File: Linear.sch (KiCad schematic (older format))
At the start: 61 parts, among them Q10 D45H11, Q11 MMBT3904, Q12 PZT3904, Q8 4403, Q9 2N7002PW, U1 OPA2376AID, U2 LM358M, U3 LM393M, U4 LM393M

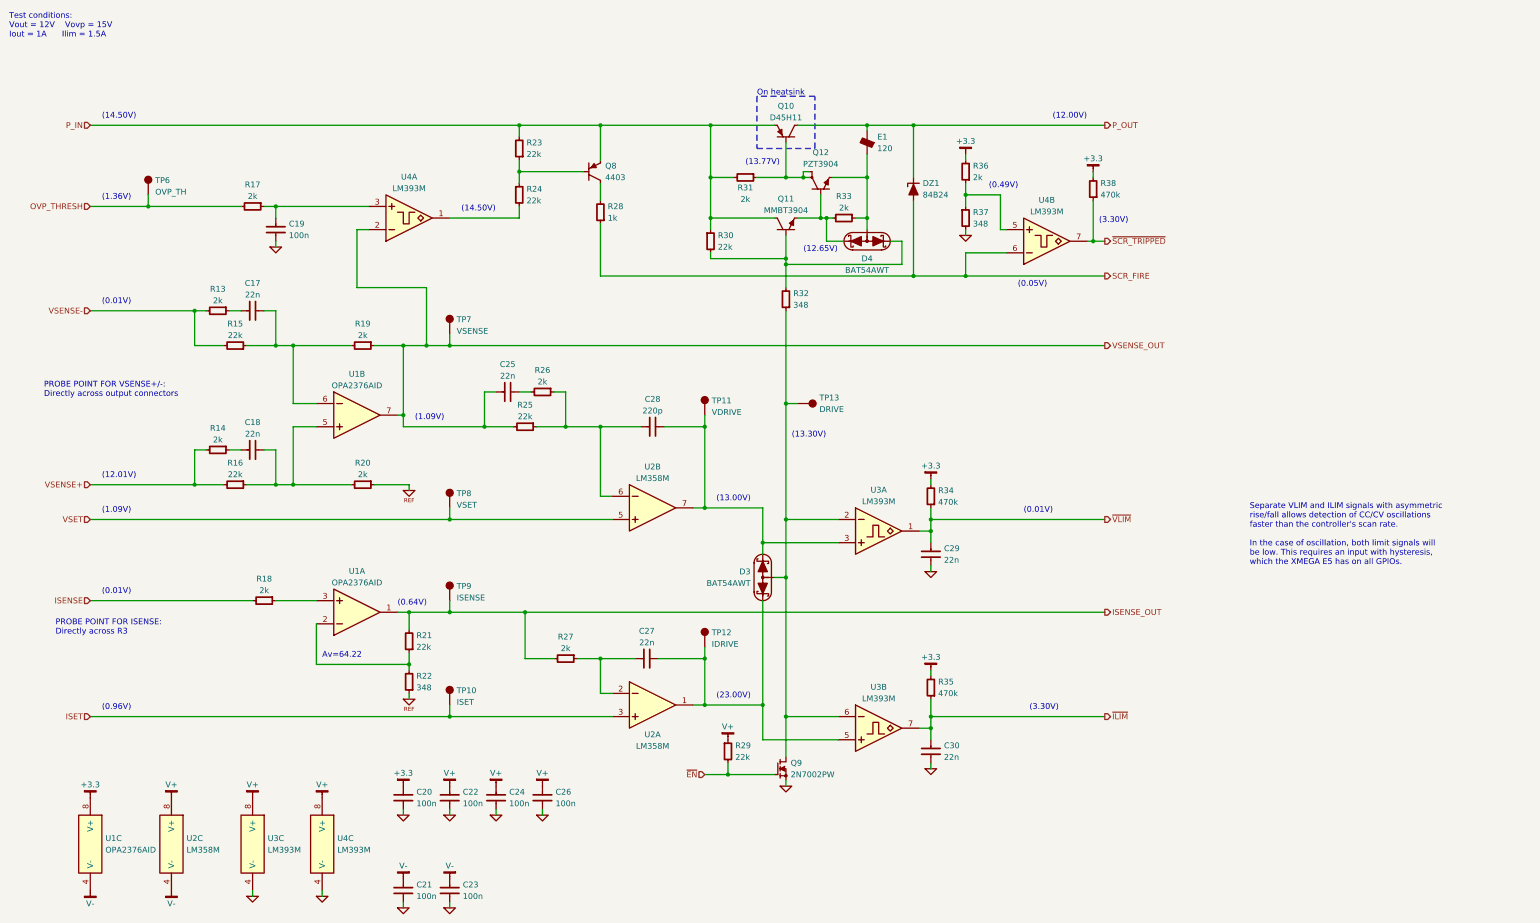
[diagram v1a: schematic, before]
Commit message: Finish PCB
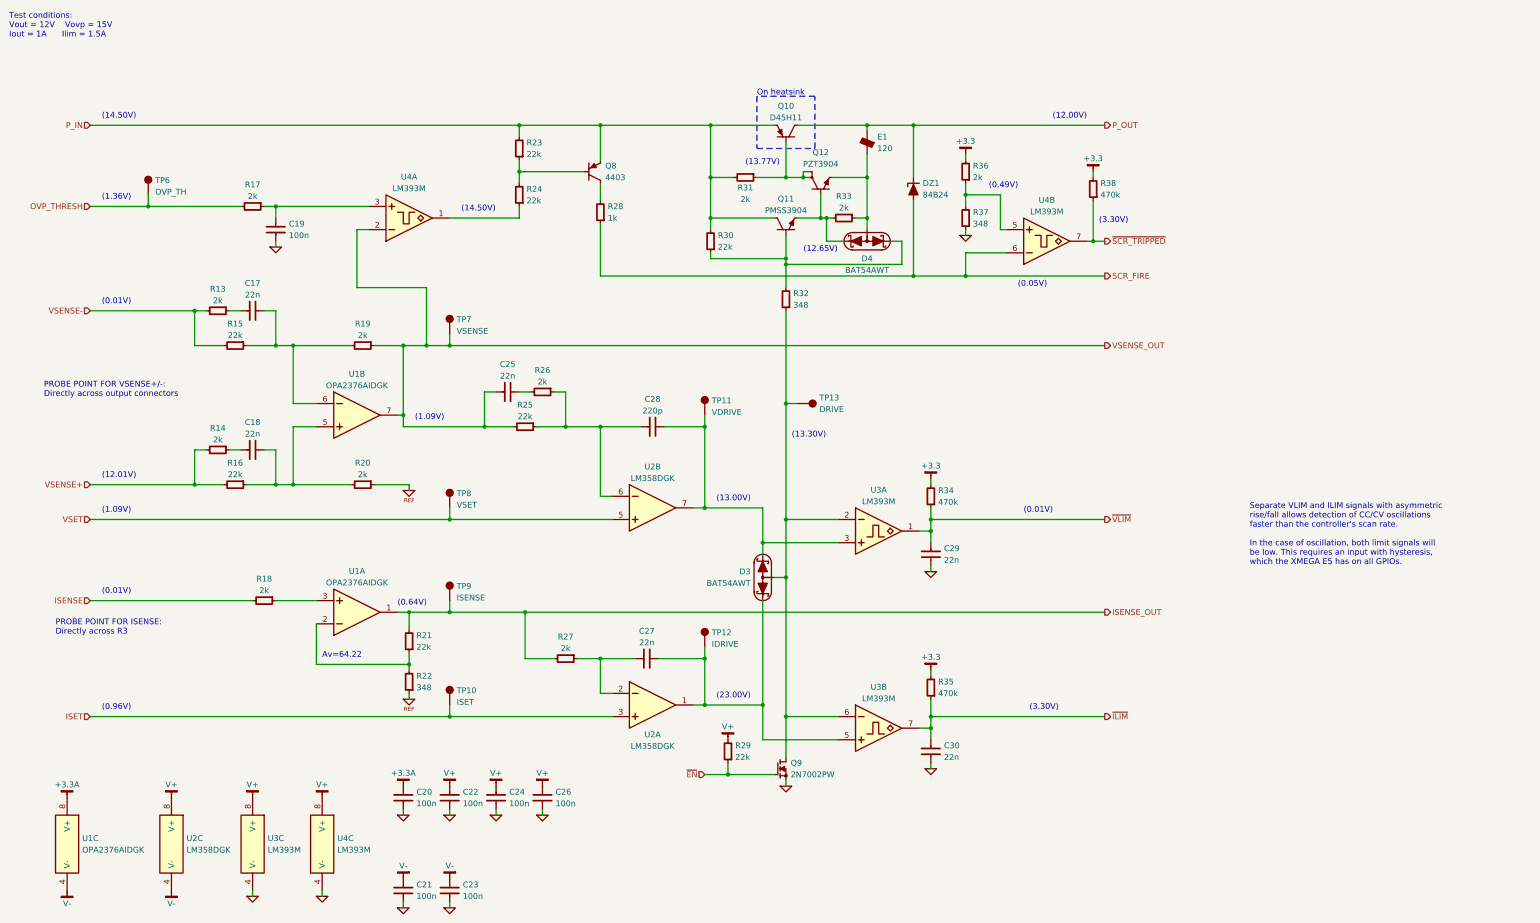
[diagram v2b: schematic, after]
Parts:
- removed C17, C18, C25, C27, C29, C30: 22n, IPC7351-Nominal:CAPC1608X55, symbol C-0603
- removed C19, C20, C21, C23: 100n, IPC7351-Nominal:CAPC1608X55, symbol C-0603
- removed C28: 220p, IPC7351-Nominal:CAPC1608X55, symbol C-0603
- removed Q11: MMBT3904, smd-semi:SOT-23, symbol MMBT3904
- removed R13, R14, R17, R18, R19, R20, R26, R27, R31, R33, R36: 2k, IPC7351-Nominal:RESC1608X50, symbol R-0603
- removed R15, R16, R21, R23, R24, R25, R29, R30: 22k, IPC7351-Nominal:RESC1608X50, symbol R-0603
- removed R22, R32, R37: 348, IPC7351-Nominal:RESC1608X50, symbol R-0603
- removed R34, R35, R38: 470k, IPC7351-Nominal:RESC1608X50, symbol R-0603
- removed U1: OPA2376AID, IPC7351-Nominal:SOIC127P600X175-8, symbol OPA2376AID
- removed U2: LM358M, IPC7351-Nominal:SOIC127P600X175-8, symbol LM358M
- added C17, C18, C25, C27, C29, C30: 22n, IPC7351-Nominal:CAPC1005X55, symbol C-0402
- added C19, C20, C21, C23: 100n, IPC7351-Nominal:CAPC1005X55, symbol C-0402
- added C28: 220p, IPC7351-Nominal:CAPC1005X55, symbol C-0402
- added Q11: PMSS3904, smd-semi:SC-70, symbol PMSS3904
- added R13, R14, R17, R18, R19, R20, R26, R27, R31, R33, R36: 2k, IPC7351-Nominal:RESC1005X40, symbol R-0402
- added R15, R16, R21, R23, R24, R25, R29, R30: 22k, IPC7351-Nominal:RESC1005X40, symbol R-0402
- added R22, R32, R37: 348, IPC7351-Nominal:RESC1005X40, symbol R-0402
- added R34, R35, R38: 470k, IPC7351-Nominal:RESC1005X40, symbol R-0402
- added U1: OPA2376AIDGK, IPC7351-Nominal:SOP65P490X110-8, symbol OPA2376AIDGK
- added U2: LM358DGK, IPC7351-Nominal:SOP65P490X110-8, symbol LM358DGK
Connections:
- net +3.3: now also R34.2, R35.2, R36.2, R38.2
- net GND: now also C19.2, C20.2, C21.2, C23.2, C29.1, C30.1, R37.1
- net ISENSE: now also R18.2
- net ISENSE_OUT: now also R21.2, R27.2, U1.1 (OUT)
- net ISET: now also U2.3 (IN+)
- net OVP_THRESH: now also R17.2
- net P_IN: now also Q11.3, R23.2, R30.2, R31.2
- net REFGND: now also R20.1, R22.1
- net V+: now also R29.2, U2.8 (V+)
- net V-: now also C21.1, C23.1, U1.4 (V-), U2.4 (V-)
- net VSENSE+: now also R14.2, R16.2
- net VSENSE-: now also R13.2, R15.2
- net VSENSE_OUT: now also C25.2, R19.1, R25.2, U1.7 (OUT)
- net VSET: now also U2.5 (IN+)
- net ~EN: now also R29.1
- net ~ILIM: now also C30.2, R35.1
- net ~SCR_TRIPPED: now also R38.1
- net ~VLIM: now also C29.2, R34.1
- net at Q10.1, Q12.2, Q12.4: now also R31.1
- net at D3.2, TP11.1, U3.3 (IN+): now also C28.1, U2.7 (OUT)
- net at D3.1, TP12.1, U3.5 (IN+): now also C27.1, U2.1 (OUT)
- net at D3.3, Q9.3, TP13.1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: now also R32.1
- net at D4.1, Q12.1: now also Q11.2, R33.2
- net at D4.3, E1.2, Q12.3: now also R33.1
- net at D4.2: now also Q11.1, R30.1, R32.2
- net at Q8.1: now also R23.1, R24.2
- net at U4.1 (OUT): now also R24.1
- net at U4.3 (IN+): now also C19.1, R17.1
- net at U4.5 (IN+): now also R36.1, R37.2
- new net: C18.1, R16.1, R20.2, U1.5 (IN+)
- new net: C17.1, R15.1, R19.2, U1.6 (IN-)
- new net: R21.1, R22.2, U1.2 (IN-)
- new net: R18.1, U1.3 (IN+)
- new net: C28.2, R25.1, R26.1, U2.6 (IN-)
- new net: C27.2, R27.1, U2.2 (IN-)
- new net: C25.1, R26.2
- new net: C17.2, R13.1
- new net: C18.2, R14.1
- new net +3.3A: C20.1, U1.8 (V+)
